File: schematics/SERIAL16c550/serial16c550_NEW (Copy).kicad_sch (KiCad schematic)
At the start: 31 parts, among them J1 DE9_Plug, U1 16550, U2 DTE, U4 74LS138, U6 PAL20L8, X1 4.915200MHz

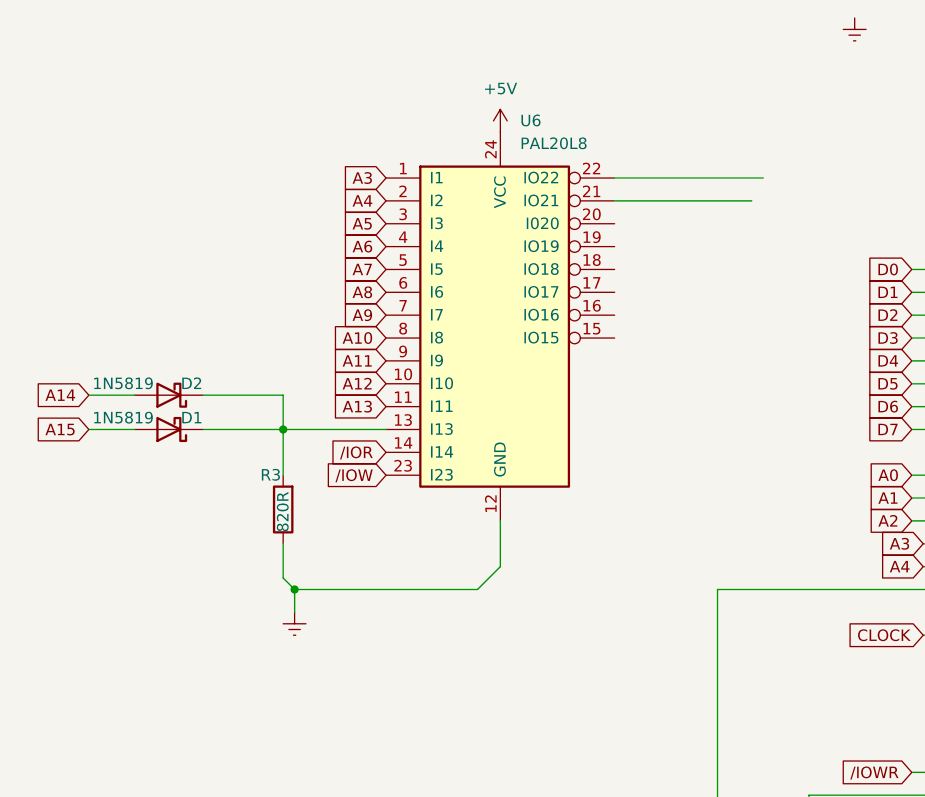
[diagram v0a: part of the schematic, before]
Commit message: Updating schematics
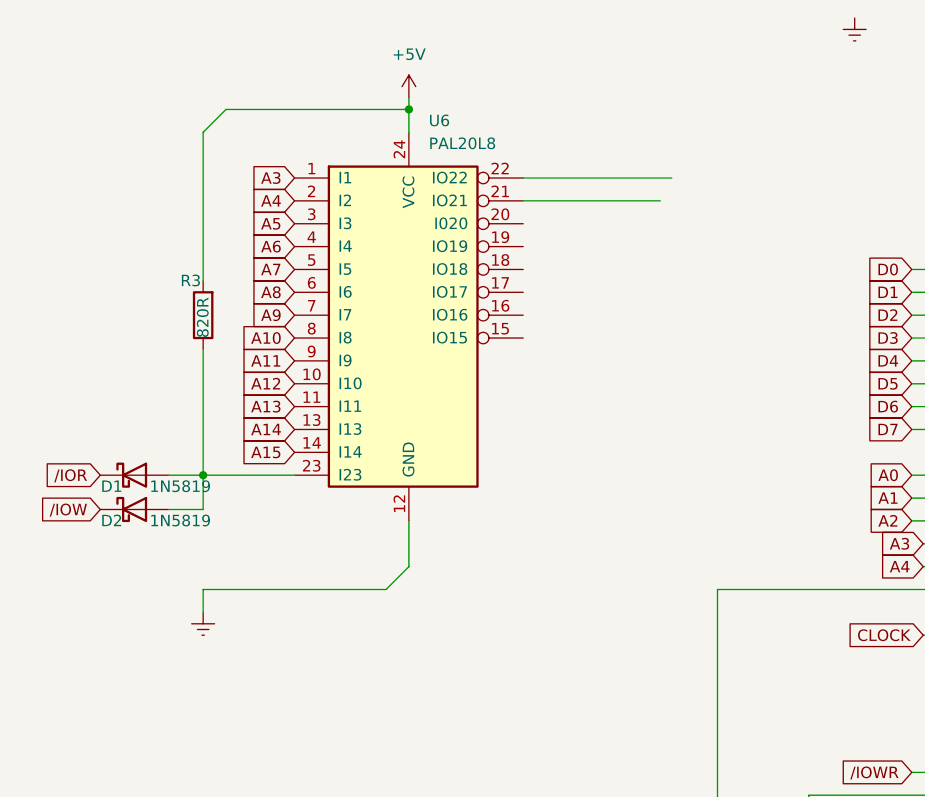
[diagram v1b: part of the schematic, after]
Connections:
- net +5V: now also R3.2
- net A14: now also U6.13 (I13); no longer D2.2 (A)
- net A15: now also U6.14 (I14); no longer D1.2 (A)
- net GNDREF: no longer R3.1
- net /IOR: now also D1.1 (K); no longer U6.14 (I14)
- net /IOW: now also D2.1 (K); no longer U6.23 (I23)
- new net: D1.2 (A), D2.2 (A), R3.1, U6.23 (I23)
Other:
- moved on the sheet: D1, D2, R3, U6
